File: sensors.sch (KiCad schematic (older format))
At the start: 14 parts, among them U4 LSM6DS3, U5 HTS221

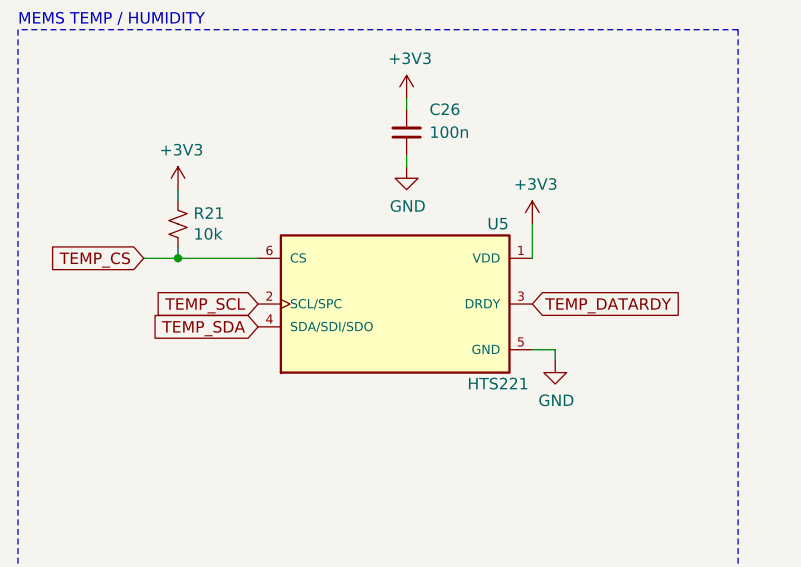
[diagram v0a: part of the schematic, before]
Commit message: update
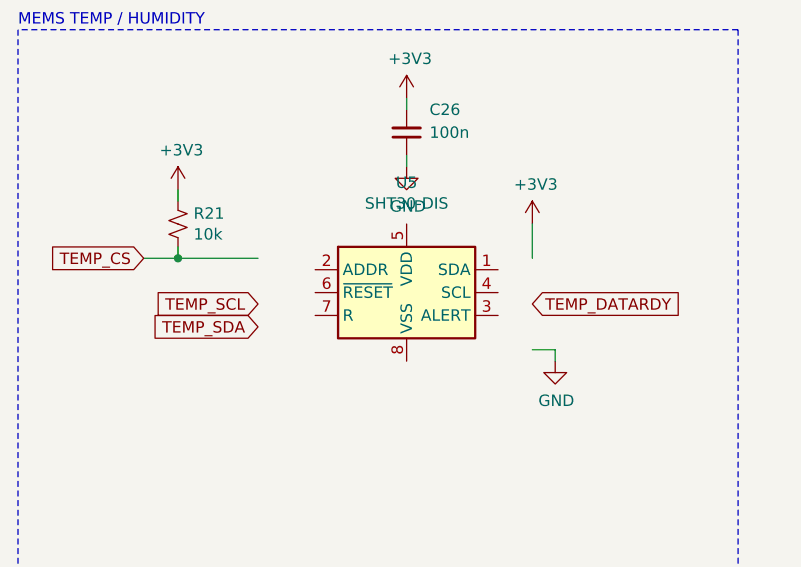
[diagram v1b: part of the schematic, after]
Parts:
- removed U5: HTS221, HTS221:XDCR_HTS221, symbol HTS221:HTS221
- added U5: SHT30-DIS, Sensor_Humidity:Sensirion_DFN-8-1EP_2.5x2.5mm_P0.5mm_EP1.1x1.7mm, symbol Sensor_Humidity:SHT30-DIS
- U4: Field4 (none) -> C967633
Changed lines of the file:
@@
 F 2 "Package_LGA:LGA-14_3x2.5mm_P0.5mm_LayoutBorder3x4y" H 2500 1600 50  0001 L CNN
 F 3 "www.st.com/resource/en/datasheet/lsm6ds3.pdf" H 3000 1650 50  0001 C CNN
+F 4 "C967633" H 2900 2300 50  0001 C CNN "Field4"
 	1    2900 2300
 	1    0    0    -1
@@
 MEMS TEMP / HUMIDITY\n\n\n
 $Comp
-L HTS221:HTS221 U5
-U 1 1 616EB7A3
-P 2450 4750
-F 0 "U5" H 2900 5100 50  0000 C CNN
-F 1 "HTS221" H 2900 4400 50  0000 C CNN
-F 2 "HTS221:XDCR_HTS221" H 2450 4750 50  0001 L BNN
-F 3 "" H 2450 4750 50  0001 L BNN
-F 4 "STMicroelectronics" H 2450 4750 50  0001 L BNN "MANUFACTURER"
-F 5 "Rev 1" H 2450 4750 50  0001 L BNN "PARTREV"
-F 6 "Manufacturer Recommendations" H 2450 4750 50  0001 L BNN "STANDARD"
-	1    2450 4750
-	1    0    0    -1
-$EndComp
-$Comp
 L power:GND #PWR060
 U 1 1 616ECBA9
@@
 Wire Notes Line
 	3950 3550 800  3550
+$Comp
+L Sensor_Humidity:SHT30-DIS U5
+U 1 1 6176112E
+P 2500 4700
+F 0 "U5" H 2500 5181 50  0000 C CNN
+F 1 "SHT30-DIS" H 2500 5090 50  0000 C CNN
+F 2 "Sensor_Humidity:Sensirion_DFN-8-1EP_2.5x2.5mm_P0.5mm_EP1.1x1.7mm" H 2500 4750 50  0001 C CNN
+F 3 "https://www.sensirion.com/fileadmin/user_upload/customers/sensirion/Dokumente/2_Humidity_Sensors/Datasheets/Sensirion_Humidity_Sensors_SHT3x_Datasheet_digital.pdf" H 2500 4750 50  0001 C CNN
+	1    2500 4700
+	1    0    0    -1
+$EndComp
 $EndSCHEMATC
